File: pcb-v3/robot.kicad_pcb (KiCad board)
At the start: 2 copper layers, 34.9 x 69.2 mm, 27 parts, among them J1 M1 PWR, J11 MB CTRL, J12 MA CTRL, J2 M2 PWR, J3 Power Connector, J4 BATT, J5 TB6612_Motor_Driver, J7 PWR, Q1 2N3904, Q2 2N3904, U2 L7805, U3 L78L33_TO92

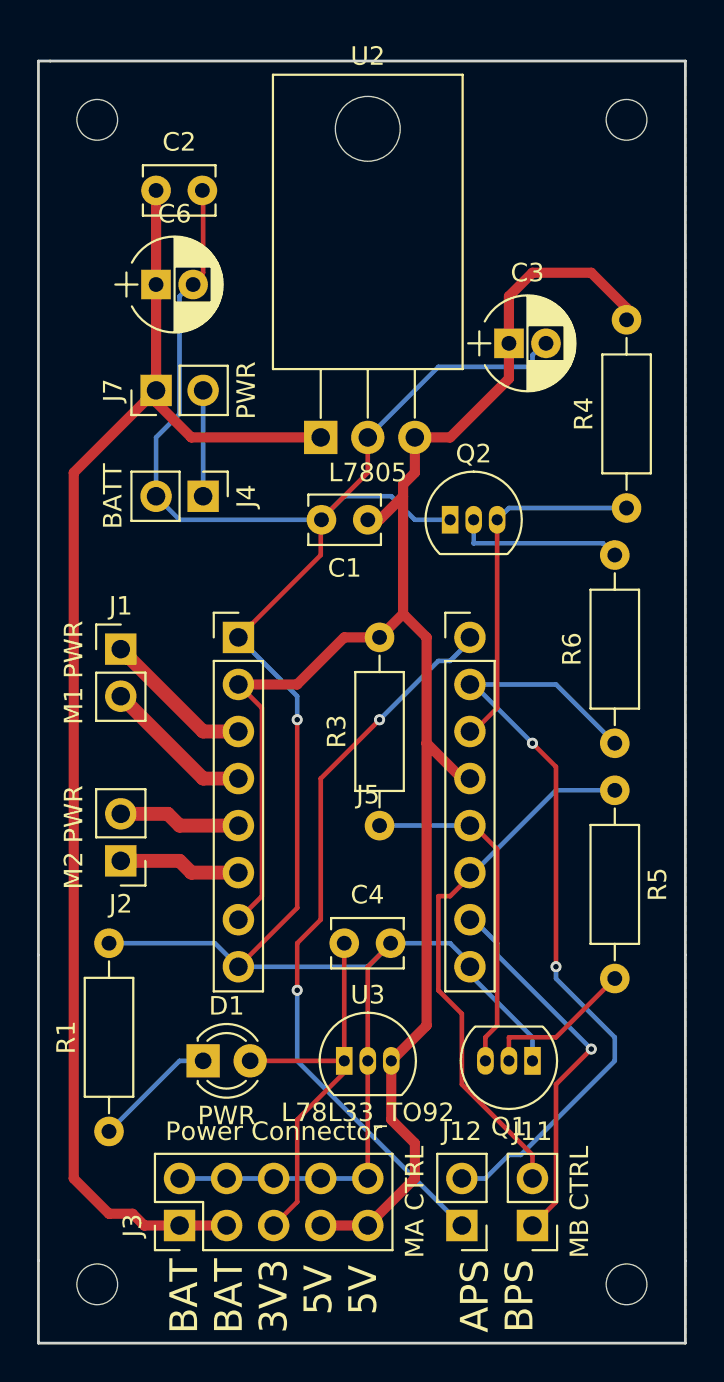
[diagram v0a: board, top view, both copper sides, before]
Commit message: small fixes
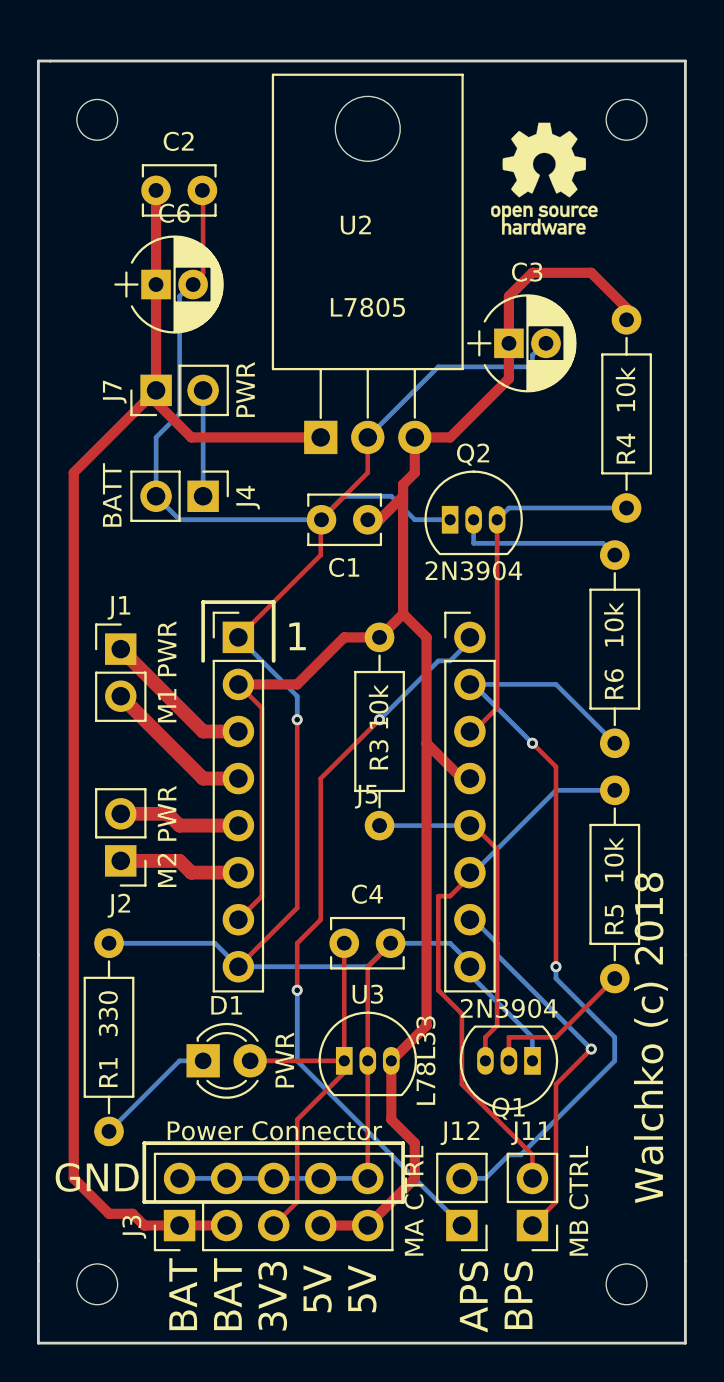
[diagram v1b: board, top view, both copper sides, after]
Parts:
- added ?: , Symbols:OSHW-Logo_5.7x6mm_SilkScreen, F.Cu at (123.2, 35.6)
- U3: value L78L33_TO92 -> L78L33
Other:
- board text added: "1"
- board text added: "GND"
- board text added: "Walchko (c) 2018"
